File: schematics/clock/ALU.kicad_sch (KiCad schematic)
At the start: 0 parts

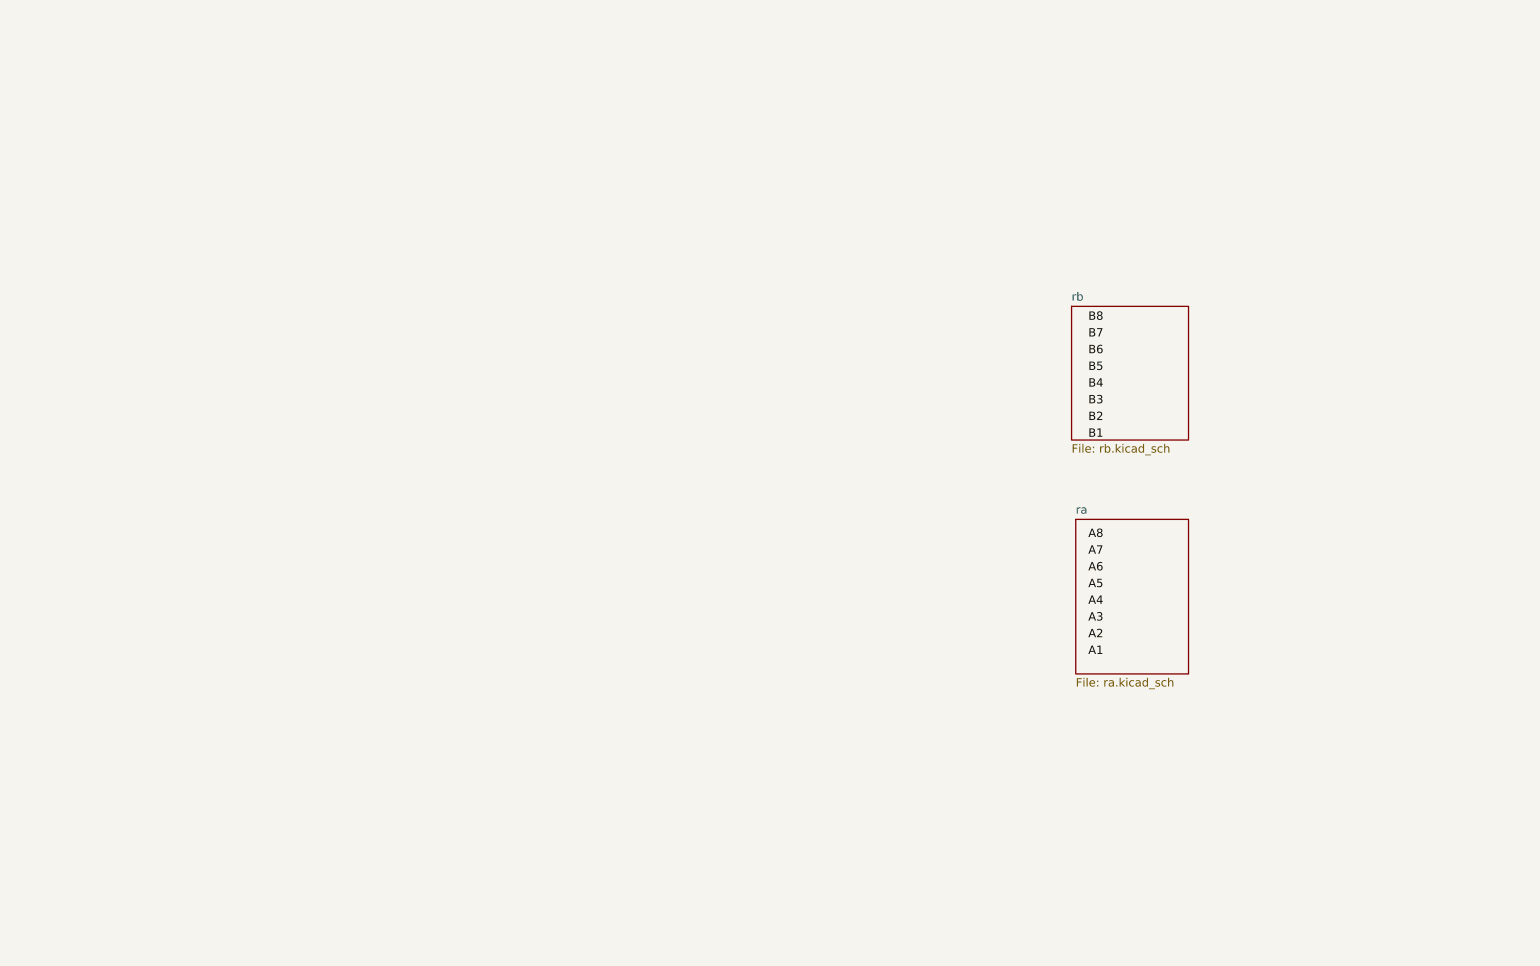
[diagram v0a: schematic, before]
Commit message: add alu
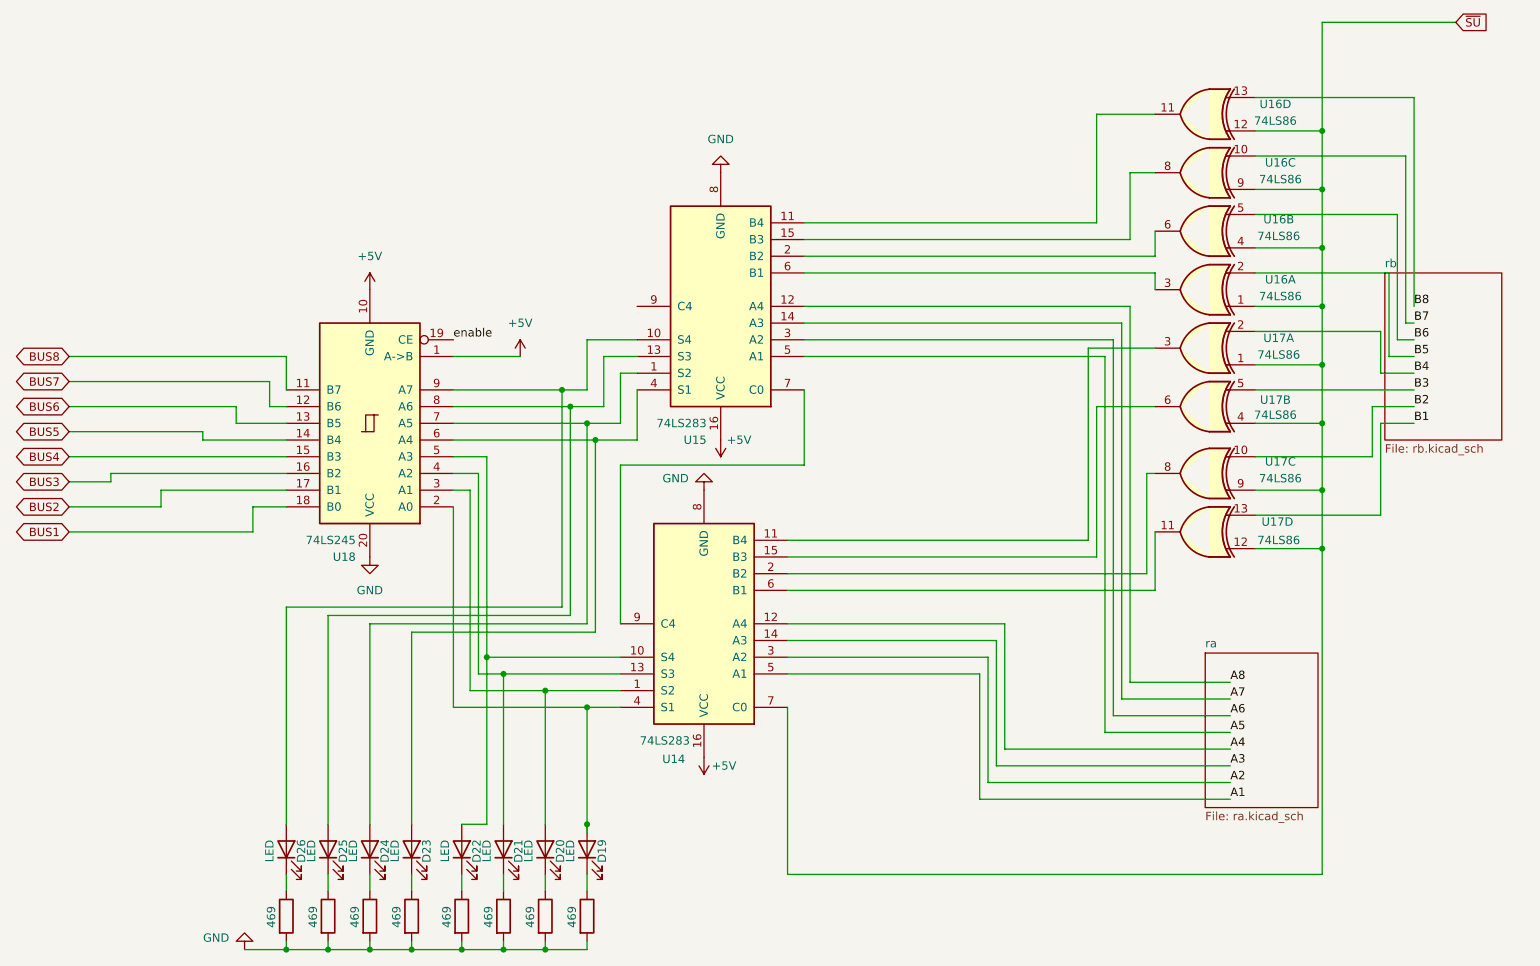
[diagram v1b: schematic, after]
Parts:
- added D19, D20, D21, D22, D23, D24, D25, D26: LED, symbol Device:LED
- added RLED26, RLED27, RLED28, RLED29, RLED30, RLED31, RLED32, RLED33: 469, symbol Device:R
- added U14, U15: 74LS283, symbol 74xx:74LS283
- added U16, U17: 74LS86, symbol 74xx:74LS86
- added U18: 74LS245, symbol 74xx:74LS245
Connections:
- net A1: now also U14.5 (A1)
- net A2: now also U14.3 (A2)
- net A3: now also U14.14 (A3)
- net A4: now also U14.12 (A4)
- net A5: now also U15.5 (A1)
- net A6: now also U15.3 (A2)
- net A7: now also U15.14 (A3)
- net A8: now also U15.12 (A4)
- net B1: now also U17.13
- net B2: now also U17.10
- net B3: now also U17.5
- net B4: now also U17.2
- net B5: now also U16.2
- net B6: now also U16.5
- net B7: now also U16.10
- net B8: now also U16.13
- new net: U14.6 (B1), U17.11
- new net: U14.15 (B3), U17.6
- new net: U15.15 (B3), U16.8
- new net: D26.1 (K), RLED33.1
- new net: D26.2 (A), U15.10 (S4), U18.9 (A7)
- new net: D23.1 (K), RLED30.1
- new net: D23.2 (A), U15.4 (S1), U18.6 (A4)
- new net: D22.1 (K), RLED29.1
- new net: D22.2 (A), U14.10 (S4), U18.5 (A3)
- new net: D19.2 (A), U14.4 (S1), U18.2 (A0)
- new net: D20.2 (A), U14.1 (S2), U18.3 (A1)
- new net: D21.2 (A), U14.13 (S3), U18.4 (A2)
- new net: D24.2 (A), U15.1 (S2), U18.7 (A5)
- new net: D25.2 (A), U15.13 (S3), U18.8 (A6)
- new net: U14.2 (B2), U17.8
- new net: U15.6 (B1), U16.3
- new net: D25.1 (K), RLED32.1
- new net: D21.1 (K), RLED28.1
- new net: D24.1 (K), RLED31.1
- new net: D19.1 (K), RLED26.1
- new net: U14.11 (B4), U17.3
- new net: U14.9 (C4), U15.7 (C0)
- new net: U15.11 (B4), U16.11
- new net: U15.2 (B2), U16.6
- new net: D20.1 (K), RLED27.1
- new net +5V: U14.16 (VCC), U15.16 (VCC), U18.1 (A->B), U18.10 (GND)
- new net BUS1: U18.18 (B0)
- new net BUS2: U18.17 (B1)
- new net BUS3: U18.16 (B2)
- new net BUS4: U18.15 (B3)
- new net BUS5: U18.14 (B4)
- new net BUS6: U18.13 (B5)
- new net BUS7: U18.12 (B6)
- new net BUS8: U18.11 (B7)
- new net GND: RLED26.2, RLED27.2, RLED28.2, RLED29.2, RLED30.2, RLED31.2, RLED32.2, RLED33.2, U14.8 (GND), U15.8 (GND), U18.20 (VCC)
- new net enable: U18.19 (CE)
- new net ~{SU}: U14.7 (C0), U16.1, U16.12, U16.4, U16.9, U17.1, U17.12, U17.4, U17.9

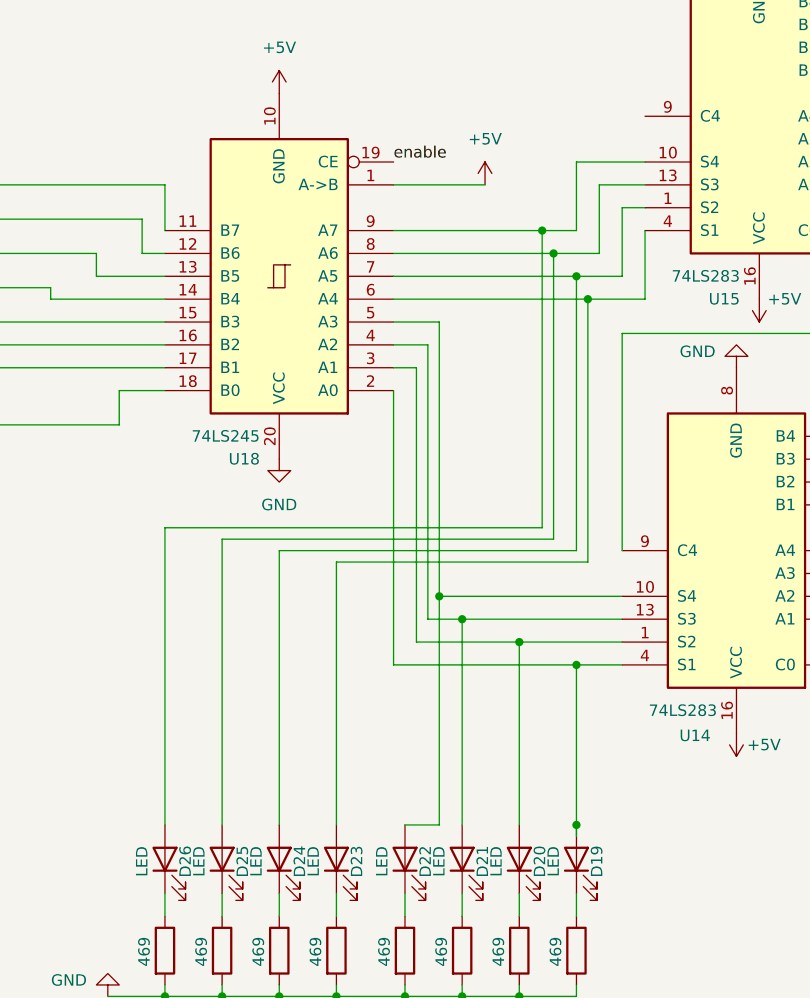
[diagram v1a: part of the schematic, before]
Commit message: fix usb 2
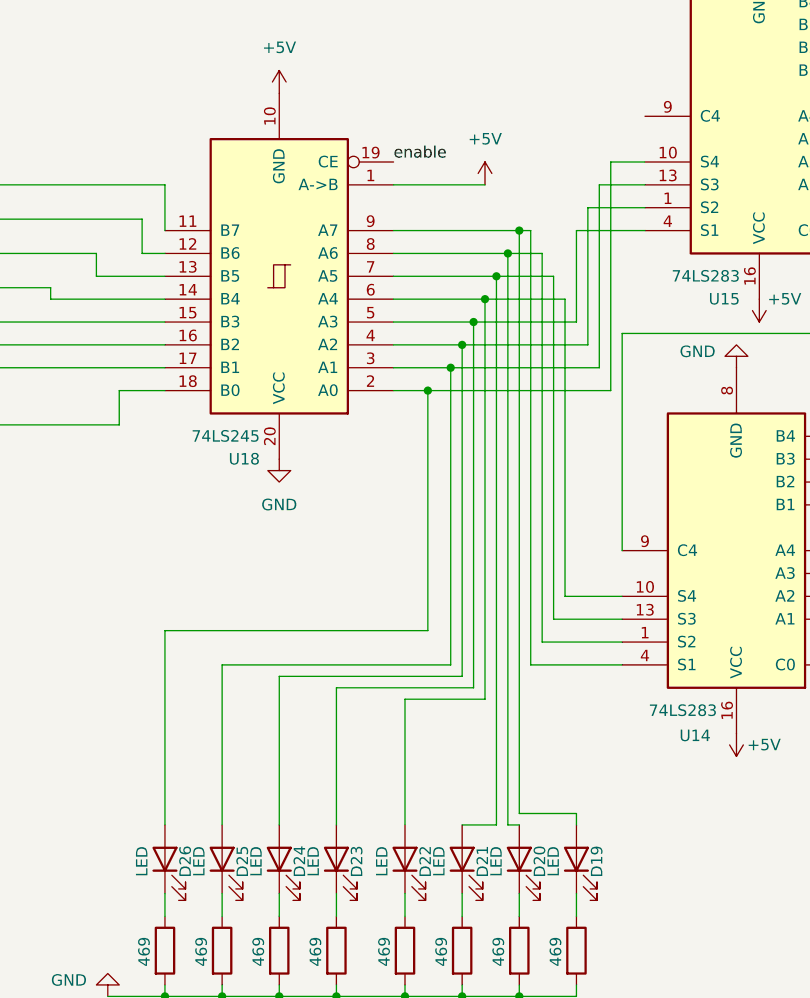
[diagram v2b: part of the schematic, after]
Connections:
- net at D26.2 (A), U15.10 (S4): now also U18.2 (A0); no longer U18.9 (A7)
- net at D23.2 (A), U15.4 (S1): now also U18.5 (A3); no longer U18.6 (A4)
- net at D22.2 (A), U14.10 (S4): now also U18.6 (A4); no longer U18.5 (A3)
- net at D19.2 (A), U14.4 (S1): now also U18.9 (A7); no longer U18.2 (A0)
- net at D20.2 (A), U14.1 (S2): now also U18.8 (A6); no longer U18.3 (A1)
- net at D21.2 (A), U14.13 (S3): now also U18.7 (A5); no longer U18.4 (A2)
- net at D24.2 (A), U15.1 (S2): now also U18.4 (A2); no longer U18.7 (A5)
- net at D25.2 (A), U15.13 (S3): now also U18.3 (A1); no longer U18.8 (A6)
